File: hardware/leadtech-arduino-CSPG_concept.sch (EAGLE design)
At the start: 41 parts, among them IC3 4050D, J9 CON_HEADER_1X02-PTH, Q1 16Mhz, U1 DS1302, U3 PL2303HX

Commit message: made some rev on dwg and schematic
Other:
- note added: "*GizDuino X 1281 equivalent pins"
- note added: "10"
- note added: "11"
- note added: "12"
- note added: "13"
- note added: "20"
- note added: "21"
- note added: "4"
- note added: "9"
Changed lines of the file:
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@@
 <?xml version="1.0" encoding="utf-8"?>
 <!DOCTYPE eagle SYSTEM "eagle.dtd">
-<eagle version="9.4.2">
+<eagle version="9.1.3">
 <drawing>
 <settings>
@@
 <text x="477.52" y="91.44" size="3.81" layer="94" ratio="12" align="bottom-center">OLED DISPLAY</text>
 <text x="480.06" y="27.94" size="3.81" layer="94" ratio="12" align="bottom-center">PIEZO BEEPER</text>
+<text x="358.14" y="55.88" size="1.778" layer="98" align="center">21</text>
+<text x="358.14" y="58.42" size="1.778" layer="98" align="center">20</text>
+<text x="350.52" y="55.88" size="1.778" layer="98" align="center">4</text>
+<text x="359.664" y="114.046" size="1.778" layer="98" align="center">9</text>
+<text x="359.664" y="109.22" size="1.778" layer="98" align="center">12</text>
+<text x="359.664" y="106.68" size="1.778" layer="98" align="center">11</text>
+<text x="359.664" y="104.14" size="1.778" layer="98" align="center">13</text>
+<text x="359.664" y="101.6" size="1.778" layer="98" align="center">10</text>
+<text x="388.62" y="20.32" size="1.778" layer="98" align="center">*GizDuino X 1281 equivalent pins</text>
 </plain>
 <instances>

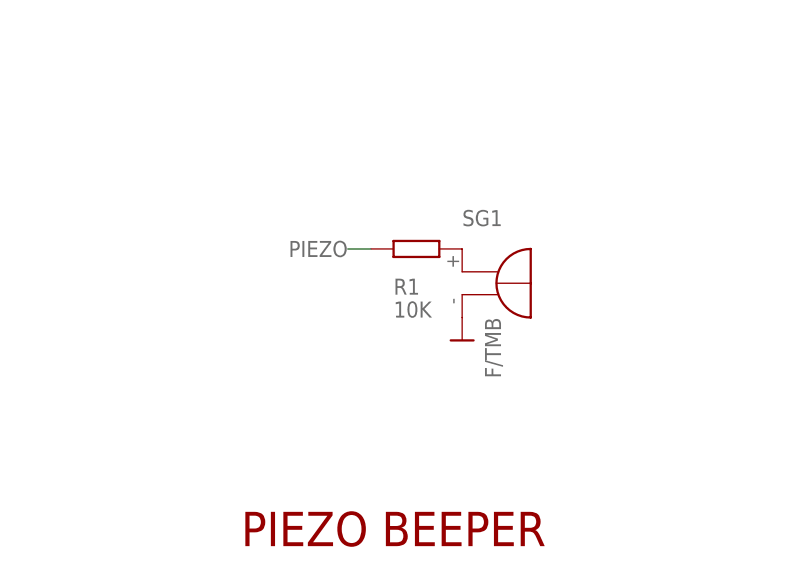
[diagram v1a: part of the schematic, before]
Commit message: update files
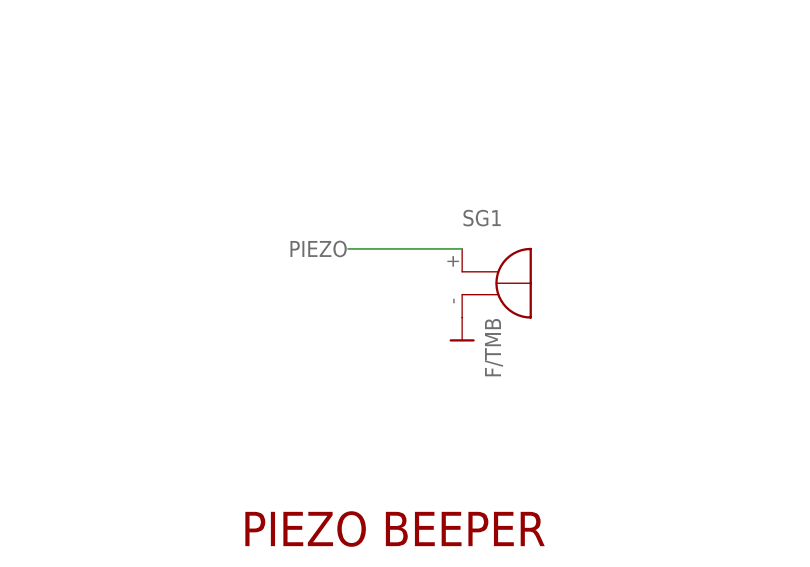
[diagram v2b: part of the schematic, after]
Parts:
- removed R1: 10K, rcl:R-EU_R0603
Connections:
- removed net N$1: R1.2, SG1.+
- net PIEZO: now also SG1.+; no longer R1.1
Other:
- note added: "2"
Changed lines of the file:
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@@
 <?xml version="1.0" encoding="utf-8"?>
 <!DOCTYPE eagle SYSTEM "eagle.dtd">
-<eagle version="9.1.3">
+<eagle version="9.4.2">
 <drawing>
 <settings>
@@
 <part name="+5V4" library="dp_devices.v6" deviceset="SUPPLY_+5V" device=""/>
 <part name="SG1" library="buzzer" library_urn="urn:adsk.eagle:library:113" deviceset="F/TMB" device="" package3d_urn="urn:adsk.eagle:package:5260/1"/>
-<part name="R1" library="rcl" library_urn="urn:adsk.eagle:library:334" deviceset="R-EU_" device="R0603" package3d_urn="urn:adsk.eagle:package:23555/3" value="10K"/>
 <part name="GND2" library="dp_devices.v6" deviceset="SUPPLY_GND" device=""/>
 <part name="MOD2" library="trosh_devices.eagle.v9" deviceset="OLED_I2C_1.3" device=""/>
@@
 <text x="359.664" y="101.6" size="1.778" layer="98" align="center">10</text>
 <text x="388.62" y="20.32" size="1.778" layer="98" align="center">*GizDuino X 1281 equivalent pins</text>
+<text x="350.52" y="93.98" size="1.778" layer="98" align="center">2</text>
 </plain>
 <instances>
@@
 <attribute name="NAME" x="487.68" y="63.5" size="1.778" layer="95"/>
 <attribute name="VALUE" x="490.22" y="53.34" size="1.778" layer="96" rot="R270"/>
-</instance>
-<instance part="R1" gate="G$1" x="482.6" y="60.96" smashed="yes">
-<attribute name="NAME" x="480.06" y="55.88" size="1.778" layer="95"/>
-<attribute name="VALUE" x="480.06" y="53.34" size="1.778" layer="96"/>
 </instance>
 <instance part="GND2" gate="G$1" x="487.68" y="50.8" smashed="yes"/>
@@
 </segment>
 </net>
-<net name="N$1" class="0">
-<segment>
+<net name="PIEZO" class="0">
+<segment>
+<label x="474.98" y="60.96" size="1.778" layer="95" align="center-right"/>
 <pinref part="SG1" gate="1" pin="+"/>
-<pinref part="R1" gate="G$1" pin="2"/>
-</segment>
-</net>
-<net name="PIEZO" class="0">
-<segment>
-<pinref part="R1" gate="G$1" pin="1"/>
-<wire x1="477.52" y1="60.96" x2="474.98" y2="60.96" width="0.1524" layer="91"/>
-<label x="474.98" y="60.96" size="1.778" layer="95" align="center-right"/>
-</segment>
-<segment>
+<wire x1="474.98" y1="60.96" x2="487.68" y2="60.96" width="0.1524" layer="91"/>
+</segment>
+<segment>

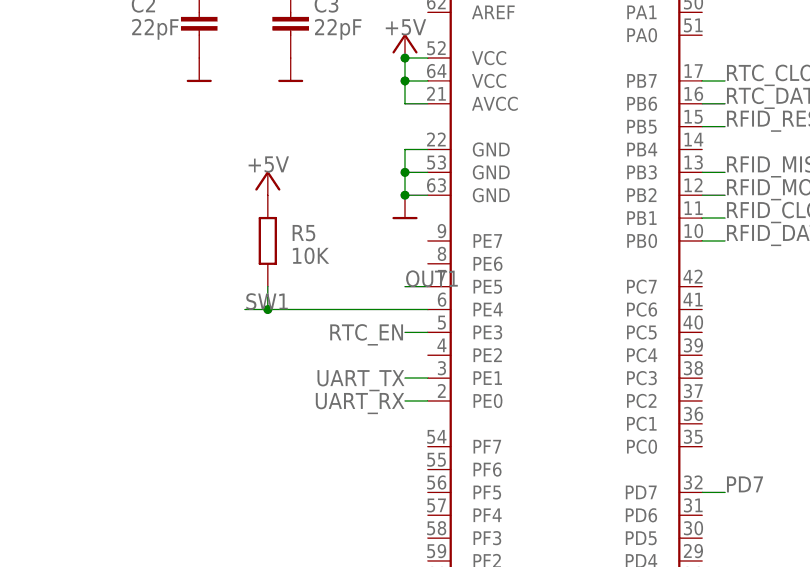
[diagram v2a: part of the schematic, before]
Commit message: small updates
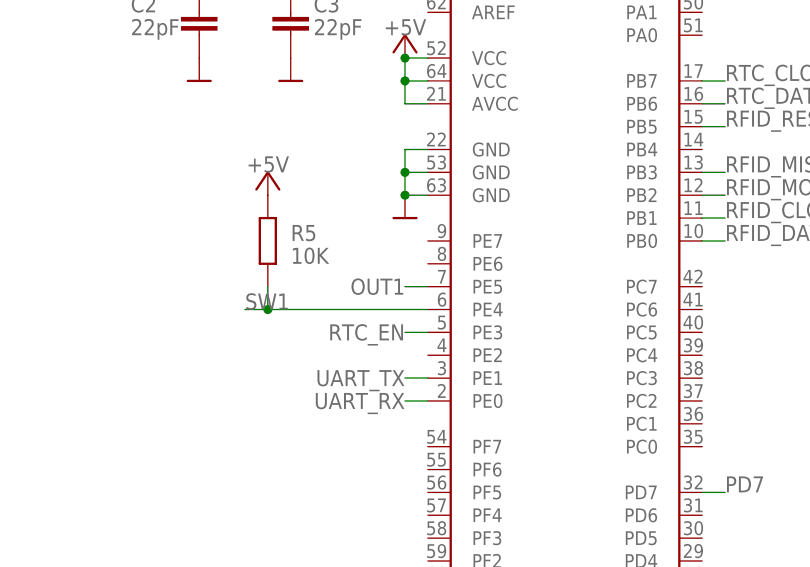
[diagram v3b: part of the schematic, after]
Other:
- note added: "3"
- note added: "PRINTER RX - 3 (PE5)"
- note added: "PRINTER TX - 2 (PE4)"
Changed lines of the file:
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@@
 <text x="388.62" y="20.32" size="1.778" layer="98" align="center">*GizDuino X 1281 equivalent pins</text>
 <text x="350.52" y="93.98" size="1.778" layer="98" align="center">2</text>
+<text x="350.52" y="96.52" size="1.778" layer="98" align="center">3</text>
+<text x="304.8" y="93.98" size="1.778" layer="98" align="center">PRINTER TX - 2 (PE4)</text>
+<text x="304.8" y="96.52" size="1.778" layer="98" align="center">PRINTER RX - 3 (PE5)</text>
 </plain>
 <instances>
@@
 <pinref part="U$1" gate="U" pin="PE5"/>
 <wire x1="340.36" y1="96.52" x2="337.82" y2="96.52" width="0.1524" layer="91"/>
-<label x="337.82" y="96.52" size="1.778" layer="95"/>
-</segment>
-</net>
+<label x="337.82" y="96.52" size="1.778" layer="95" align="center-right"/>
+</segment>
+</net>

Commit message: add gizduino pins on schematic, add bug comment on value of month on vendor firmware, add time sketches
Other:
- note added: "5"
- note added: "6"
- note added: "7"
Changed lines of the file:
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@@
 <text x="304.8" y="93.98" size="1.778" layer="98" align="center">PRINTER TX - 2 (PE4)</text>
 <text x="304.8" y="96.52" size="1.778" layer="98" align="center">PRINTER RX - 3 (PE5)</text>
+<text x="359.664" y="119.126" size="1.778" layer="98" align="center">7</text>
+<text x="359.664" y="116.586" size="1.778" layer="98" align="center">6</text>
+<text x="350.52" y="91.44" size="1.778" layer="98" align="center">5</text>
 </plain>
 <instances>
